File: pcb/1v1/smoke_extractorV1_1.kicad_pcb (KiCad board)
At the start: 2 copper layers, 80 x 29 mm, 55 parts, among them IC1 DW01A, J1 Conn_01x01_Socket, J2 Conn_01x01_Socket, Q1 FDN336P, SW1 SW_Push, U1 USB-TYPE-C-31-M-15, U2 SDDJE, U3 LM324DT, U5 TP4056, U7 ME2149FM5G, U8 FH8205

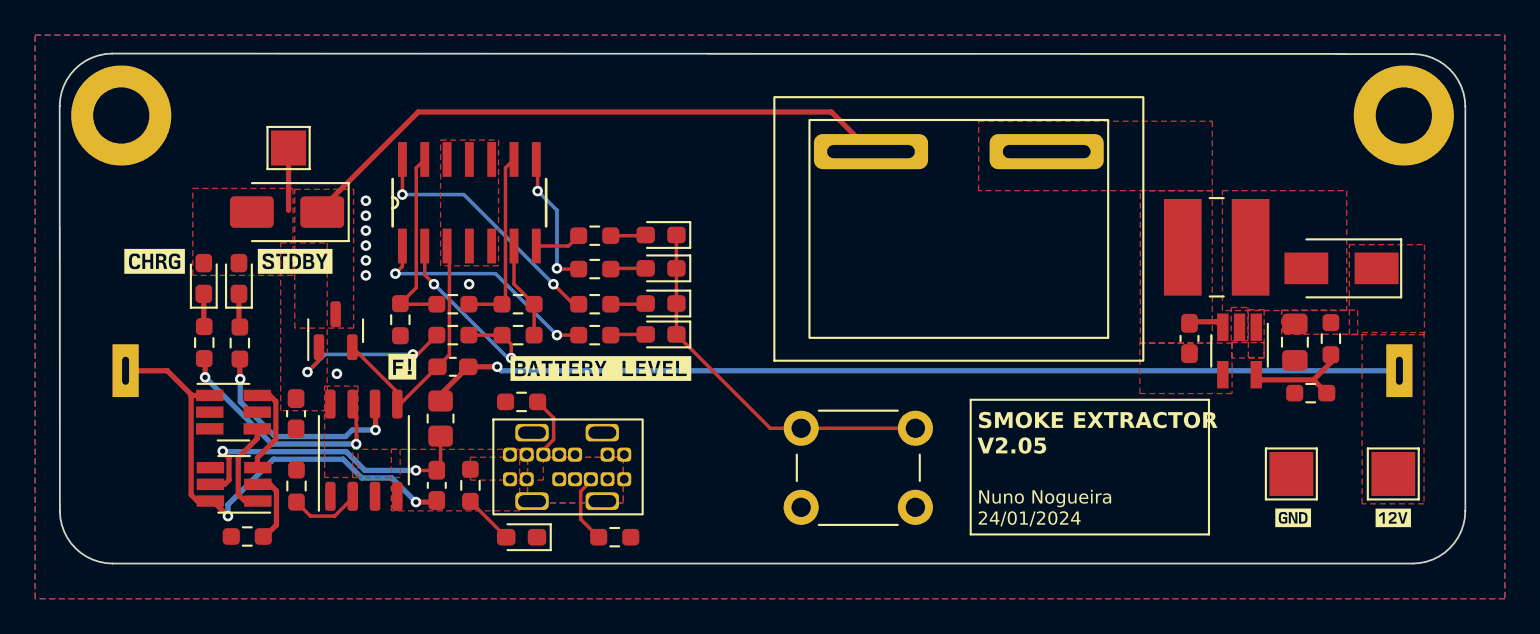
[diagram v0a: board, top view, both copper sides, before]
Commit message: more changes.
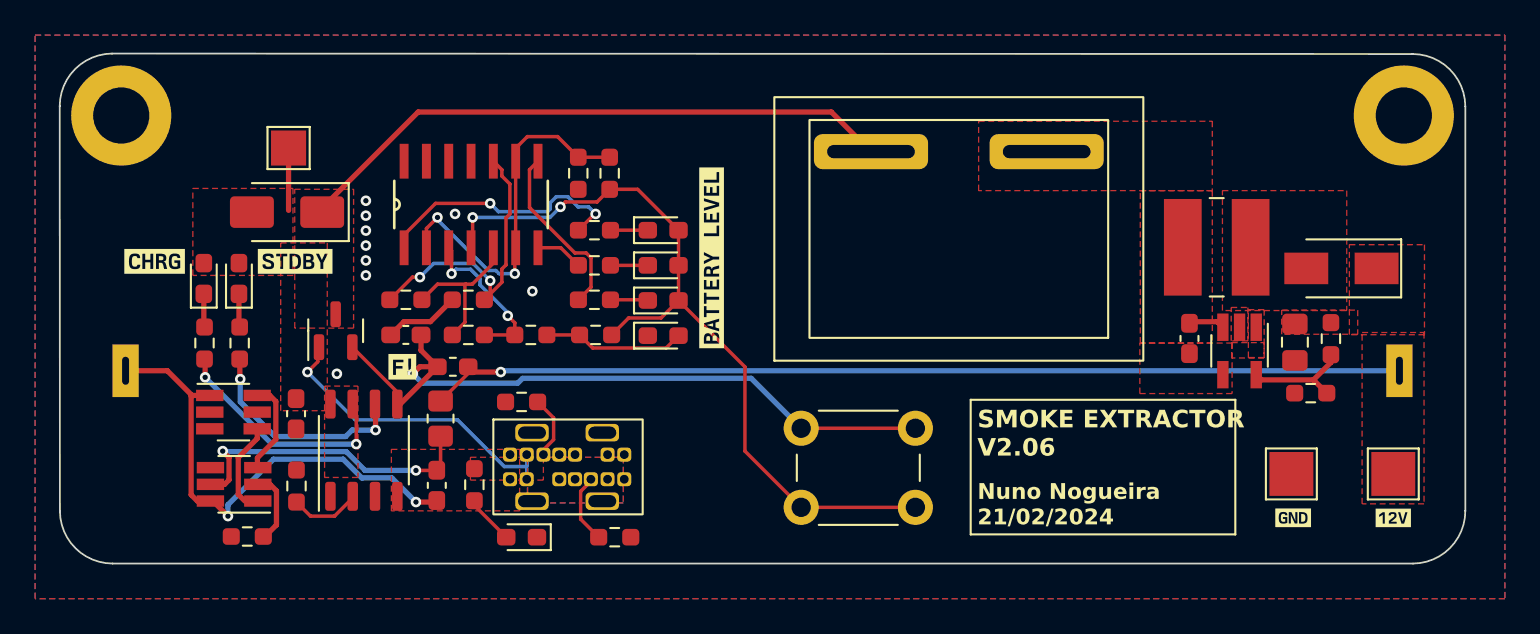
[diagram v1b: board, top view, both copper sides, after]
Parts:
- removed D6: RLED, LED_SMD:LED_0603_1608Metric_Pad1.05x0.95mm_HandSolder
- removed R19: 1k, Resistor_SMD:R_0603_1608Metric_Pad0.98x0.95mm_HandSolder
- added C2: 0.1u, Capacitor_SMD:C_0603_1608Metric_Pad1.08x0.95mm_HandSolder, F.Cu at (83.6, 81.9)
- added D9: RLED, LED_SMD:LED_0603_1608Metric_Pad1.05x0.95mm_HandSolder, F.Cu at (98.2, 81.9)
- added R7: 3k3, Resistor_SMD:R_0603_1608Metric_Pad0.98x0.95mm_HandSolder, F.Cu at (93.4, 72.7)
- added R8: 3k3, Resistor_SMD:R_0603_1608Metric_Pad0.98x0.95mm_HandSolder, F.Cu at (72.1, 82.3)
- D2: value RLED -> YLED
- D3, D4: value RLED -> GLED
- R1: value 3k6 -> 3k3
- R11, R12, R14, R15, R18: value 1k -> 3k3
- R13: value 1k -> 4k7
- R2: value 1k -> 5k1
- moved R15 20.3 mm to (74.1, 82.3), turned to 90 degrees
- moved R18 17.4 mm to (87.5, 90.4)
- moved R11 12.7 mm to (94.3, 79.9), turned to 180 degrees
- moved kibuzzard-65B168C9 8.91 mm to (101.0, 77.5), turned to 90 degrees
- moved R1 8.13 mm to (94.4, 81.9)
- moved D4 5.93 mm to (98.2, 75.9), turned to 0 degrees
- moved R5 4.03 mm to (87.2, 79.9), turned to 0 degrees
- moved R12 3.97 mm to (94.3, 77.9), turned to 180 degrees
- moved R13 3.65 mm to (95.2, 72.7), turned to 90 degrees
- moved R3 3.33 mm to (87.2, 81.9), turned to 0 degrees
- moved R4 2.69 mm to (83.6, 79.9), turned to 0 degrees
- moved R14 2.21 mm to (94.3, 75.9), turned to 180 degrees
- moved D2 1.83 mm to (98.2, 79.9), turned to 0 degrees
- moved D3 1.73 mm to (98.2, 77.9), turned to 0 degrees
- moved R2 0.73 mm to (90.7, 81.9), turned to 180 degrees
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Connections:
- D3 pad 1: Net-(D2-K) -> Net-(D3-K)
- D3 pad 2: Net-(D3-A) -> Net-(D2-A)
- D4 pad 1: Net-(D2-K) -> Net-(D4-K)
- D4 pad 2: Net-(D4-A) -> Net-(D2-A)
- R1 pad 1: VBUS -> Net-(D9-A)
- R1 pad 2: Net-(U3-NEG_1) -> Net-(D2-A)
- R11 pad 1: VBUS -> Net-(D2-K)
- R11 pad 2: Net-(D1-A) -> Net-(U3-OUT3)
- R12 pad 1: Net-(U3-OUT1) -> Net-(D3-K)
- R12 pad 2: Net-(D4-A) -> Net-(U3-OUT2)
- R13 pad 1: Net-(U3-OUT2) -> Net-(D2-A)
- R13 pad 2: Net-(D3-A) -> Net-(U3-NEG3)
- R14 pad 1: Net-(U3-OUT3) -> Net-(D4-K)
- R14 pad 2: Net-(D2-A) -> Net-(U3-OUT1)
- R15 pad 1: Net-(U3-OUT4) -> Net-(U5-~{STDBY})
- R15 pad 2: Net-(D6-A) -> Net-(D8-K)
- R18 pad 1: Net-(D7-K) -> VBUS
- R18 pad 2: Net-(U5-~{CHRG}) -> Net-(D1-A)
- R2 pad 1: Net-(U3-NEG_1) -> Net-(D9-A)
- R2 pad 2: Net-(U3-NEG_2) -> Net-(U3-POS_1)
- R3 pad 1: Net-(U3-NEG_2) -> Net-(U3-POS_2)
- R3 pad 2: Net-(U3-NEG3) -> Net-(U3-POS_1)
- R4 pad 1: Net-(U3-NEG3) -> Net-(U3-POS_3)
- R4 pad 2: Net-(U3-NEG_4) -> Net-(U3-POS_2)
- R5 pad 1: Net-(U3-NEG_4) -> VBAT-PROTECT
- R5 pad 2: VBAT-PROTECT -> Net-(U3-POS_3)
- SW1 pad 1: VBAT-PROTECT -> Net-(D2-A)
- SW1 pad 2: Net-(D2-K) -> VBAT+PROTECT
- U3 pad 10: VBAT+PROTECT -> Net-(U3-POS_3)
- U3 pad 12: VBAT+PROTECT -> unconnected-(U3-POS_4-Pad12)
- U3 pad 13: Net-(U3-NEG_4) -> unconnected-(U3-NEG_4-Pad13)
- U3 pad 14: Net-(U3-OUT4) -> unconnected-(U3-OUT4-Pad14)
- U3 pad 2: Net-(U3-NEG_1) -> Net-(U3-NEG3)
- U3 pad 3: VBAT+PROTECT -> Net-(U3-POS_1)
- U3 pad 4: VBAT+PROTECT -> Net-(D2-A)
- U3 pad 5: VBAT+PROTECT -> Net-(U3-POS_2)
- U3 pad 6: Net-(U3-NEG_2) -> Net-(U3-NEG3)
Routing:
- net Net-(D2-A): track 2.00 -> 44.9 mm, vias 0 -> 2
- net VBAT+PROTECT: track 14.7 -> 41.3 mm, vias 0 -> 1
- net Net-(D2-K): track 21.5 -> 2.14 mm
- net Net-(U3-POS_3): track 0.00 -> 17.1 mm, vias 0 -> 2
- net Net-(U3-OUT4): track 14.6 -> 0.00 mm, vias 2 -> 0
- net Net-(U3-NEG_1): track 11.9 -> 0.00 mm, vias 2 -> 0
- net Net-(U3-NEG_4): track 10.9 -> 0.00 mm
- net Net-(U3-NEG3): track 10.4 -> 21.1 mm, vias 0 -> 2
- net Net-(U3-POS_1): track 0.00 -> 9.24 mm, vias 0 -> 2
- net Net-(U3-POS_2): track 0.00 -> 9.01 mm
- net VBUS: track 13.5 -> 22.0 mm, vias 2 -> 1
- net Net-(D9-A): track 0.00 -> 8.10 mm
- net Net-(U3-NEG_2): track 5.55 -> 0.00 mm
- net VBAT-PROTECT: track 2.07 -> 6.40 mm, vias 8 -> 9
- net Net-(U3-OUT3): track 7.94 -> 10.2 mm, vias 2 -> 0
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- removed copper zone on F.Cu, net VBAT+PROTECT
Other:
- board text added: "Nuno Nogueira 21/02/2024"
- board text added: "SMOKE EXTRACTOR V2.06"
- board text removed: "Nuno Nogueira 24/01/2024"
- board text removed: "SMOKE EXTRACTOR V2.05"
